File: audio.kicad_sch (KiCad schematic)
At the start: 33 parts, among them J1 AudioJack3, U1 CS4344-CZZ

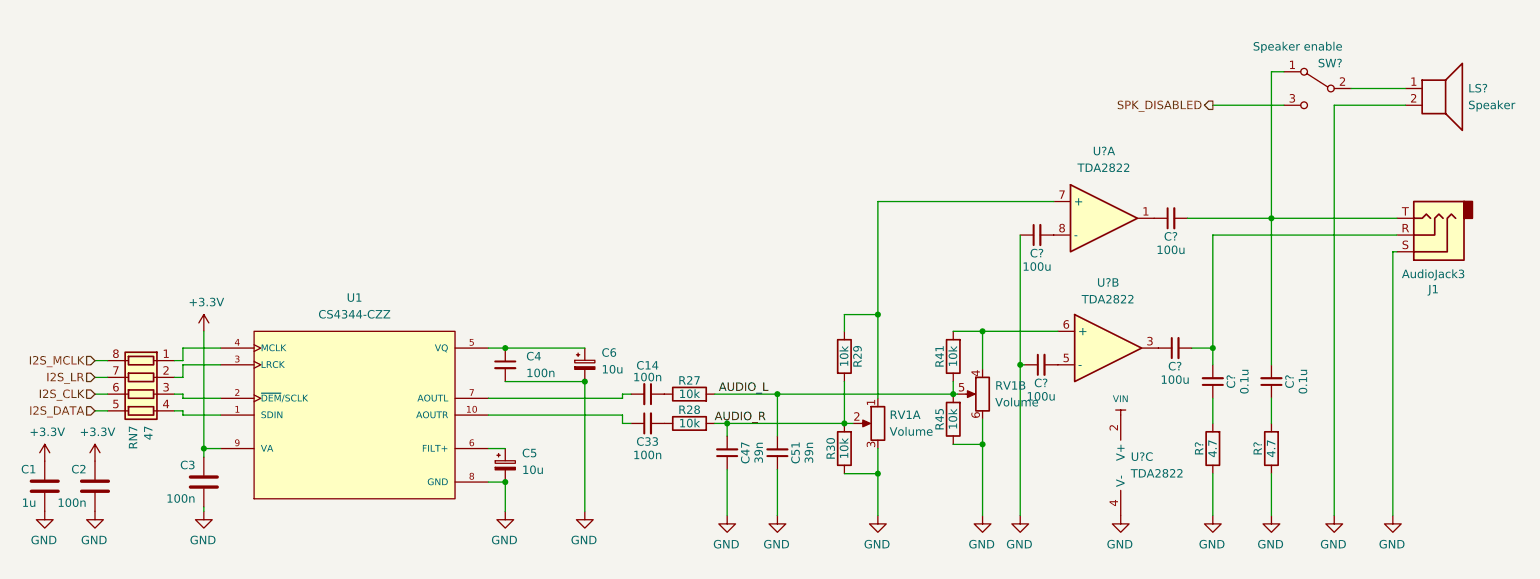
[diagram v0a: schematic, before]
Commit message: Finishing touches for audio circuit
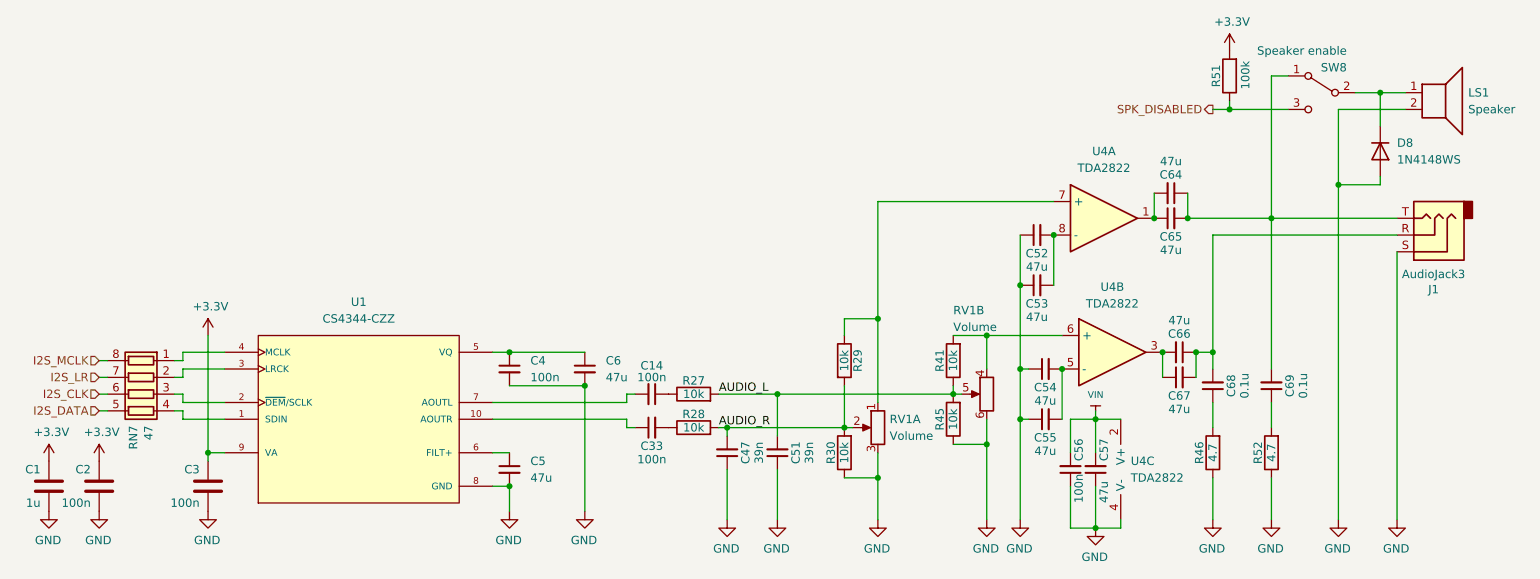
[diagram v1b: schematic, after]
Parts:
- removed C5, C6: 10u, Capacitor_SMD:C_0402_1005Metric, symbol Device:C_Polarized_Small
- added C5, C53, C55, C57, C6, C64, C67: 47u, Capacitor_SMD:C_0805_2012Metric, symbol Device:C_Small
- added C56: 100n, Capacitor_SMD:C_0603_1608Metric, symbol Device:C_Small
- added D8: 1N4148WS, Diode_SMD:D_SOD-323, symbol Diode:1N4148WS
- added R51: 100k, Resistor_SMD:R_0402_1005Metric, symbol mch2021-rescue:R-Device
- C52, C54, C65, C66: renamed from C?; value 100u -> 47u; footprint Capacitor_SMD:C_0402_1005Metric -> Capacitor_SMD:C_0805_2012Metric
- gave numbers to parts that had none: 7
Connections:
- net +3V3: now also R51.2
- net GND: now also C5.2, C53.1, C55.1, C56.1, C57.1, C6.2, D8.2 (A)
- net SPK_DISABLED: now also R51.1
- net VIN: now also C56.2, C57.2
- net at C68.2, J1.R: now also C66.1, C67.2; no longer C66.2
- net at C65.2, C69.2, J1.T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: now also C64.1
- net at LS1.1, SW8.2 (B): now also D8.1 (K)
- net at C65.1, U4.1: now also C64.2
- net at C52.2, U4.8 (-): now also C53.2
- net at C4.1, U1.5 (VQ): now also C6.1
- net at U1.6 (FILT+): now also C5.1
- net at U4.3: now also C66.2, C67.1; no longer C66.1
- net at C54.2, U4.5 (-): now also C55.2
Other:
- moved on the sheet: C1, C14, C2, C3, C33, C4, C54, C66, C68, C69, LS1, R27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
